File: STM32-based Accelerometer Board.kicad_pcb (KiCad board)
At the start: 2 copper layers, 22.6 x 13.5 mm, 12 parts, among them J1 Conn_01x04_Male, U1 ADXL345, U2 STM32F030F4Px, Y1 Crystal

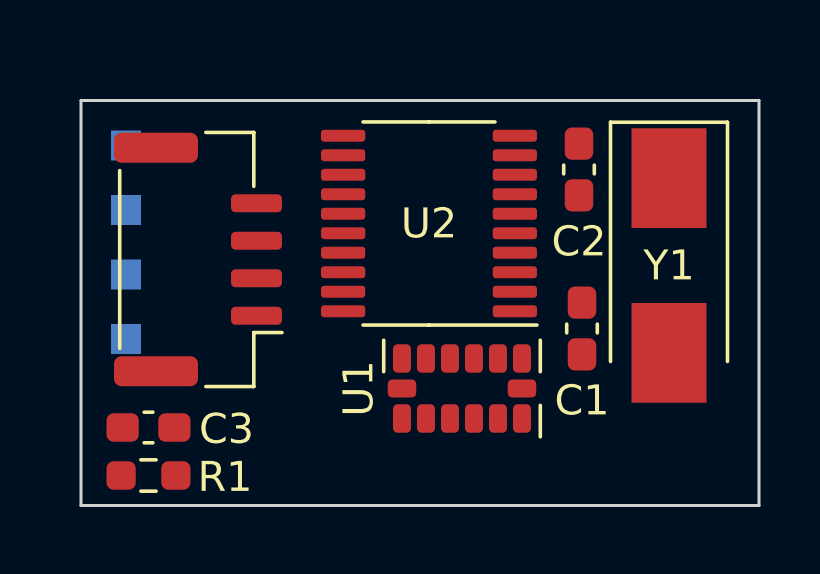
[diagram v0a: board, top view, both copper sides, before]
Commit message: Smaller! Think there's low-hanging fruit, but saving status.
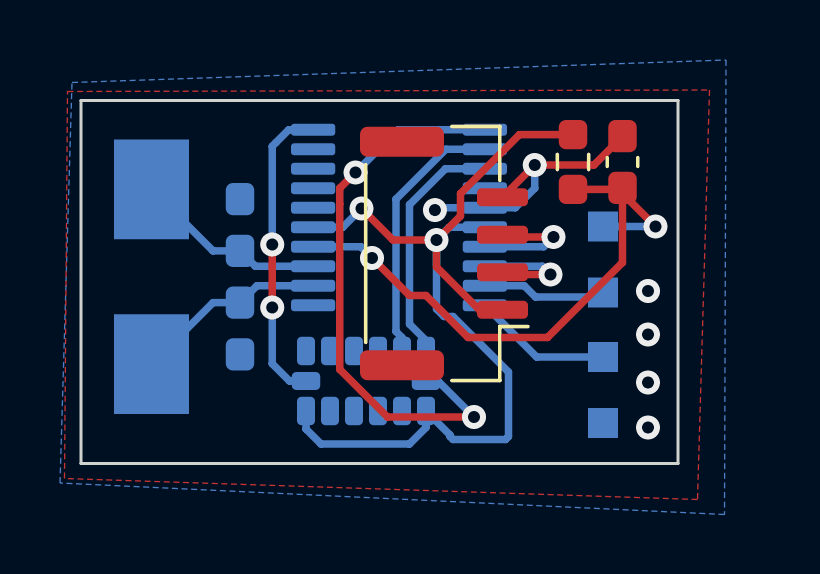
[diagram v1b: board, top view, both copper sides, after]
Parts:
- C1, C2, U1, U2, Y1: moved to B.Cu
- moved TP3 18.4 mm to (29.4, 22.8)
- moved C3 18.1 mm to (30.1, 14.1), turned to 90 degrees
- moved R1 17.6 mm to (28.4, 14.1), turned to -90 degrees
- moved Y1 17.3 mm to (14.3, 17.9)
- moved TP4 16.3 mm to (29.4, 16.2)
- moved TP1 16.1 mm to (29.4, 18.4)
- moved TP2 16.1 mm to (29.4, 20.6)
- moved C2 11.5 mm to (17.3, 16.1)
- moved C1 11.4 mm to (17.3, 19.6), turned to 90 degrees
- moved J1 8.20 mm to (24.1, 17.1)
- moved U1 3.21 mm to (21.5, 21.4)
- moved U2 1.02 mm to (22.6, 15.9), turned to 0 degrees
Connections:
- U1 pad 7: unconnected-(U1-Pad7) -> ADXL_NCS
- U2 pad 10: unconnected-(U2-Pad10) -> ADXL_NCS
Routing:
- net +3V3: track 0.00 -> 33.2 mm, vias 0 -> 2
- net NRST: track 0.00 -> 20.3 mm, vias 0 -> 2
- net SCLK: track 0.00 -> 18.9 mm, vias 0 -> 2
- net ADXL_NCS: track 0.00 -> 10.2 mm, vias 0 -> 2
- net GND: track 0.00 -> 9.25 mm, vias 0 -> 6
- net MISO: track 0.00 -> 8.80 mm
- net MOSI: track 0.00 -> 8.11 mm
- net Net-(C1-Pad2): track 0.00 -> 6.47 mm
- net Net-(C2-Pad2): track 0.00 -> 6.45 mm
- net /SWCLK: track 0.00 -> 4.65 mm
- net /SWDIO: track 0.00 -> 4.15 mm
- net SCL: track 0.00 -> 4.15 mm, vias 0 -> 1
- net SDA: track 0.00 -> 3.93 mm, vias 0 -> 1
- added copper zone on B.Cu, net GND
- added copper zone on F.Cu, net GND
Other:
- board size 22.6 x 13.5 mm -> 19.9 x 12.1 mm
